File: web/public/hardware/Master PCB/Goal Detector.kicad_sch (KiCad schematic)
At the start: 10 parts, among them U4 LM339

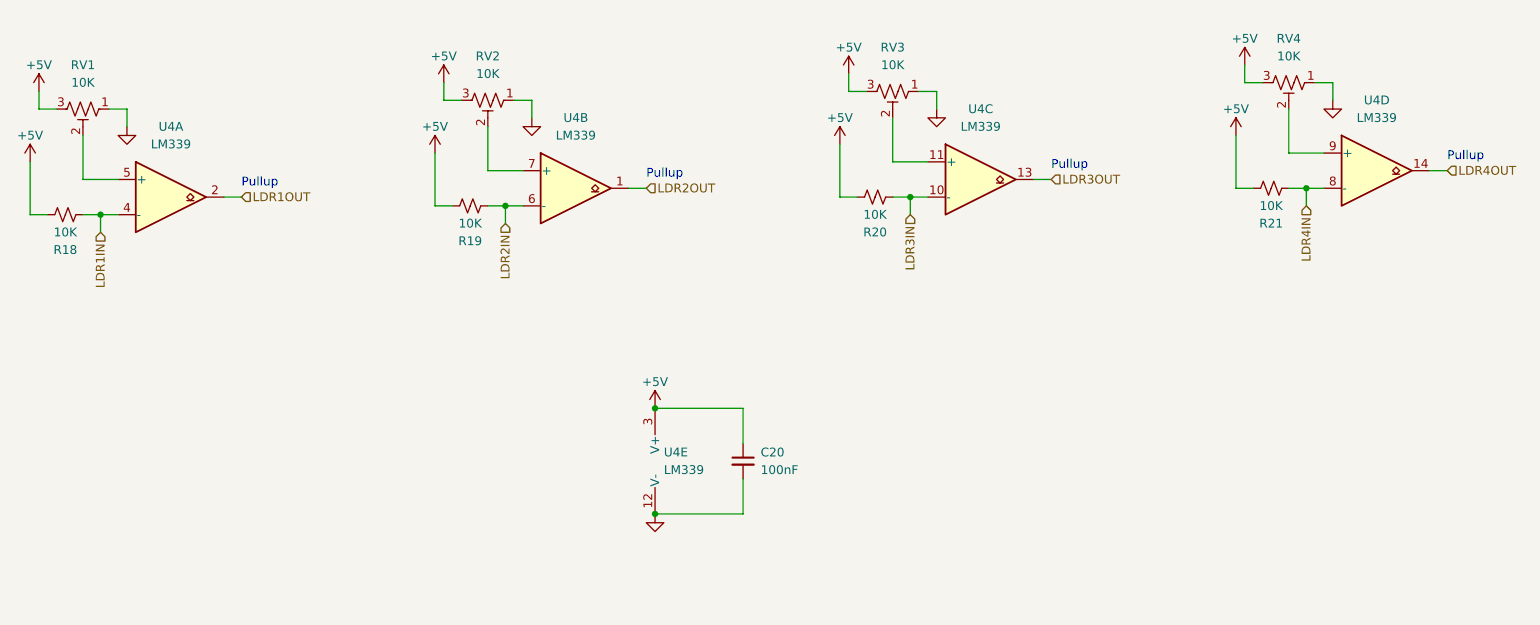
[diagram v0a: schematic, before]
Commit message: More misc. cleanup and generate updated production files
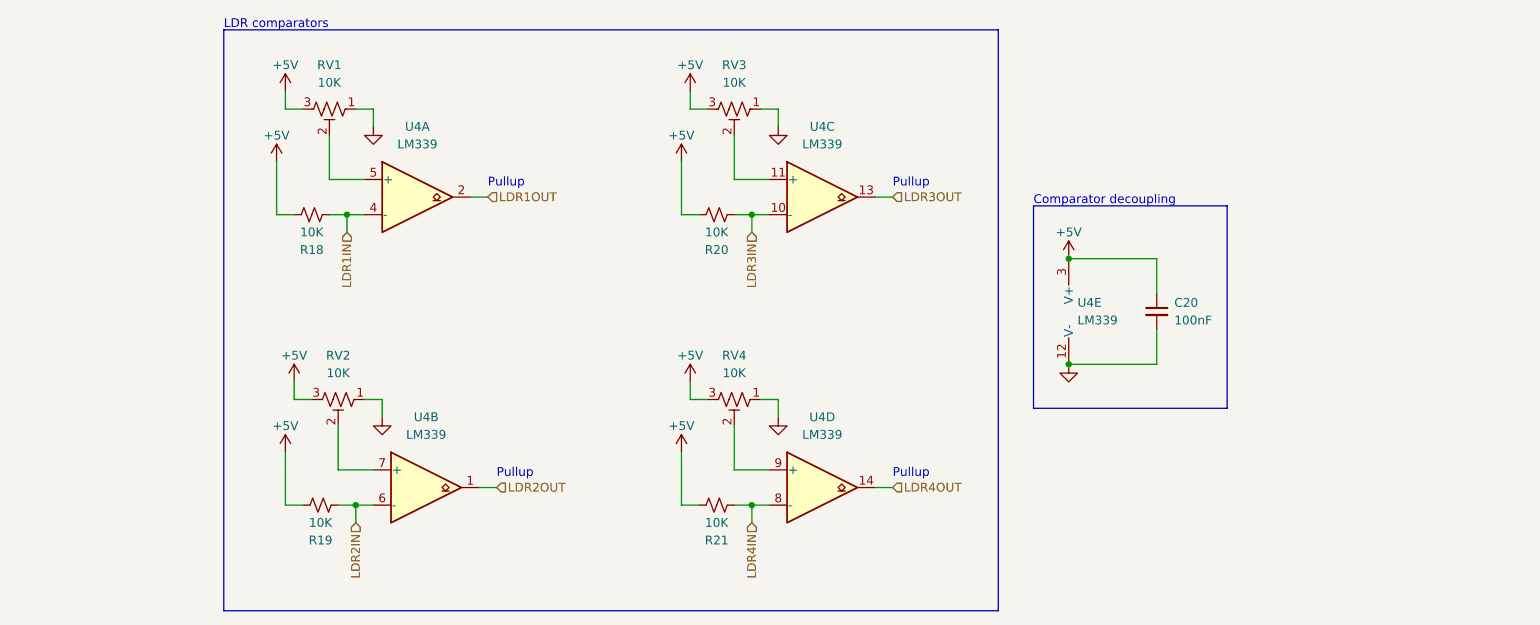
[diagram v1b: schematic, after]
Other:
- note added: "Comparator decoupling"
- note added: "LDR comparators"
- moved on the sheet: C20, R18, R19, R20, R21, RV1, RV2, RV3, RV4, U4A, U4B, U4C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
